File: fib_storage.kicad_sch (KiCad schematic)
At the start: 1 part, among them J2 Bus_M.2_Socket_M

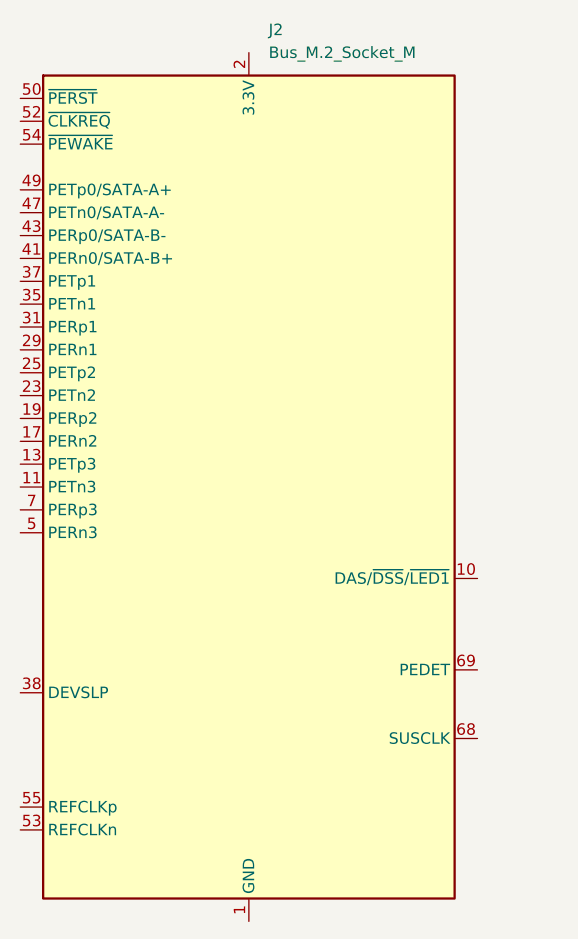
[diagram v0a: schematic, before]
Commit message: added symbol&footprint for orin/sodimm, added a bunch of specs and docs, partially implemented audio, full steam ahead
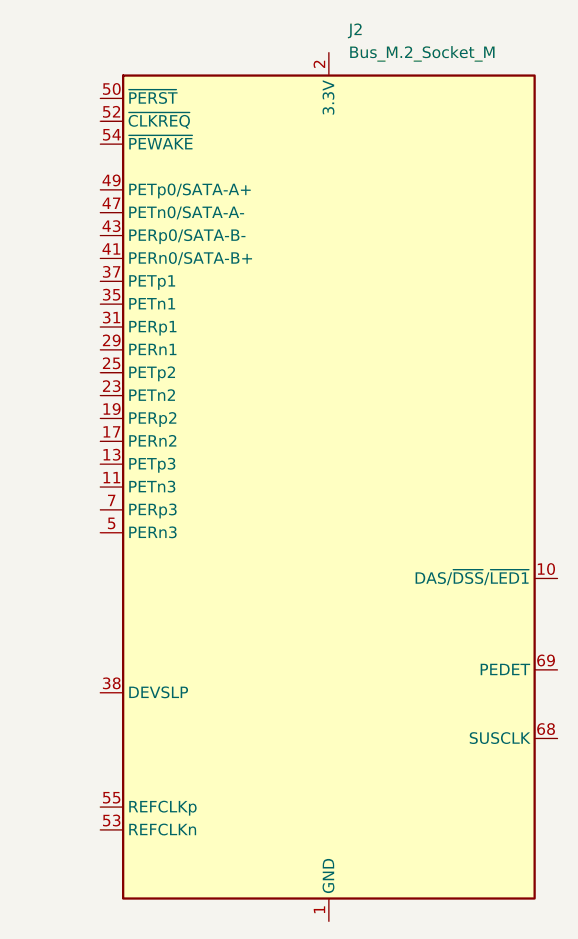
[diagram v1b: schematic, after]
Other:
- moved on the sheet: J2
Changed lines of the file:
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@@
 	(symbol
 		(lib_id "Connector:Bus_M.2_Socket_M")
-		(at 77.47 81.28 0)
+		(at 86.36 81.28 0)
 		(unit 1)
 		(exclude_from_sim no)
@@
 		(fields_autoplaced yes)
 		(property "Reference" "J2"
-			(at 79.6641 30.48 0)
+			(at 88.5541 30.48 0)
 			(effects
 				(font
@@
 		)
 		(property "Value" "Bus_M.2_Socket_M"
-			(at 79.6641 33.02 0)
+			(at 88.5541 33.02 0)
 			(effects
 				(font
@@
 		)
 		(property "Footprint" ""
-			(at 77.47 54.61 0)
+			(at 86.36 54.61 0)
 			(effects
 				(font
@@
 		)
 		(property "Datasheet" "http://read.pudn.com/downloads794/doc/project/3133918/PCIe_M.2_Electromechanical_Spec_Rev1.0_Final_11012013_RS_Clean.pdf#page=155"
-			(at 77.47 54.61 0)
+			(at 86.36 54.61 0)
 			(effects
 				(font
@@
 		)
 		(property "Description" "M.2 Socket 3 Mechanical Key M"
-			(at 77.47 81.28 0)
+			(at 86.36 81.28 0)
 			(effects
 				(font
